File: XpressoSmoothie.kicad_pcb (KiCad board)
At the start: 2 copper layers, 99.7 x 99.7 mm, 129 parts, among them J1 HEADER_4, J10 HEADER_3X2, J11 Pwr_in, J12 HEADER_4, J13 HEADER_6, J14 HEADER_3X2, J15 HEADER_4, J16 HEADER_3, J17 HEADER_3, J18 HEADER_3, J19 HEADER_2, J2 HEADER_4, J20 HEADER_2, J21 HEADER_2, J22 HEADER_2, J23 HEADER_3, J24 HEADER_3, J25 HEADER_3, J26 USB, J27 HEADER_4, J28 MICROSD-MOLEX, J29 HEADER_4, J3 HEADER_3, J30 HEADER_4, J4 HEADER_3X2, J5 HEADER_3X2, J6 LPCXPRESSO_1769_HEADER, J7 HEADER_4, J8 HEADER_4, J9 HEADER_3X2, M1 LOGO_OSHW, M2 LOGO_OSHW, Q1 IRLB 8743, Q2 IRLB 8743, Q3 IRLB 8743, Q4 IRLB 8743, SW1 SW_PUSH, SW2 SW_PUSH, SW3 SW_PUSH, U1 POLOLU_A4988, U10 TC4422A, U11 TC4422A, U12 LM1117-3.3, U2 POLOLU_A4988, U3 POLOLU_A4988, U4 POLOLU_A4988, U5 POLOLU_A4988, U7 LM7809CT, U8 TC4422A, U9 TC4422A

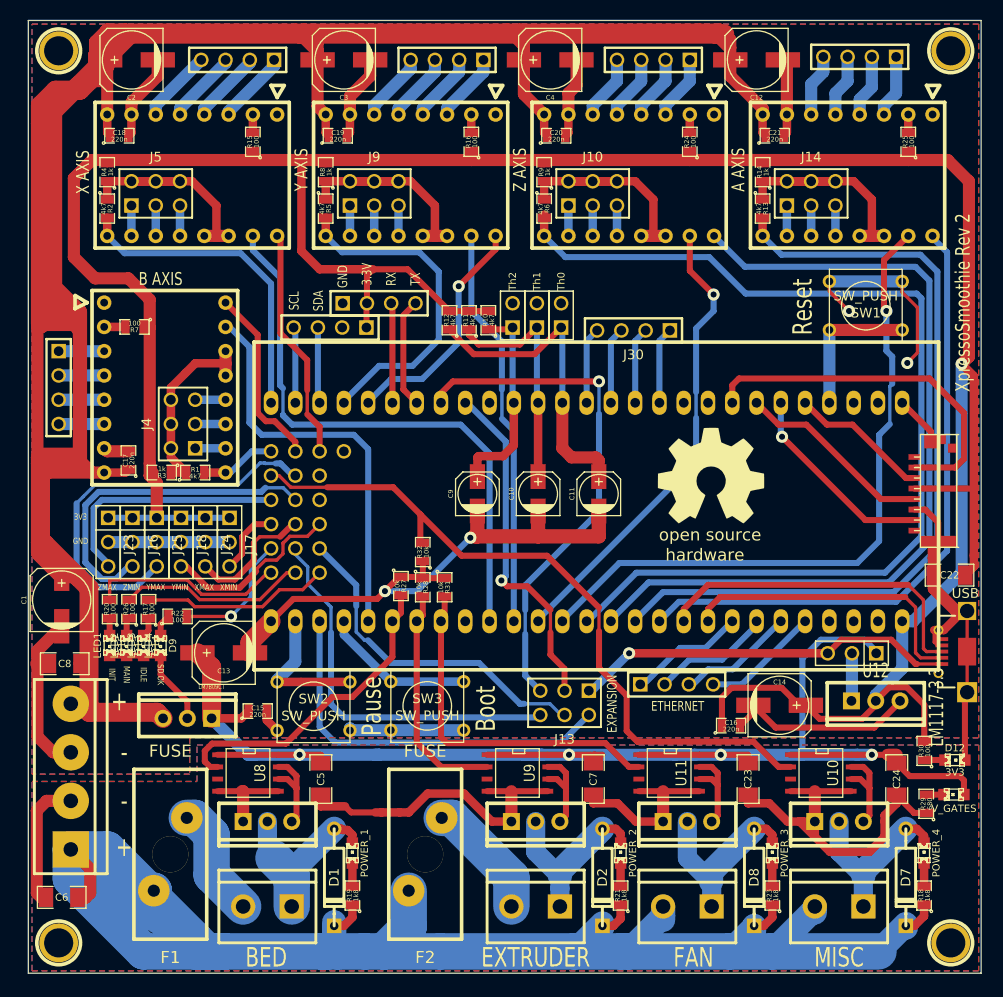
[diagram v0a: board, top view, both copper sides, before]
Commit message: Rev3 layout.
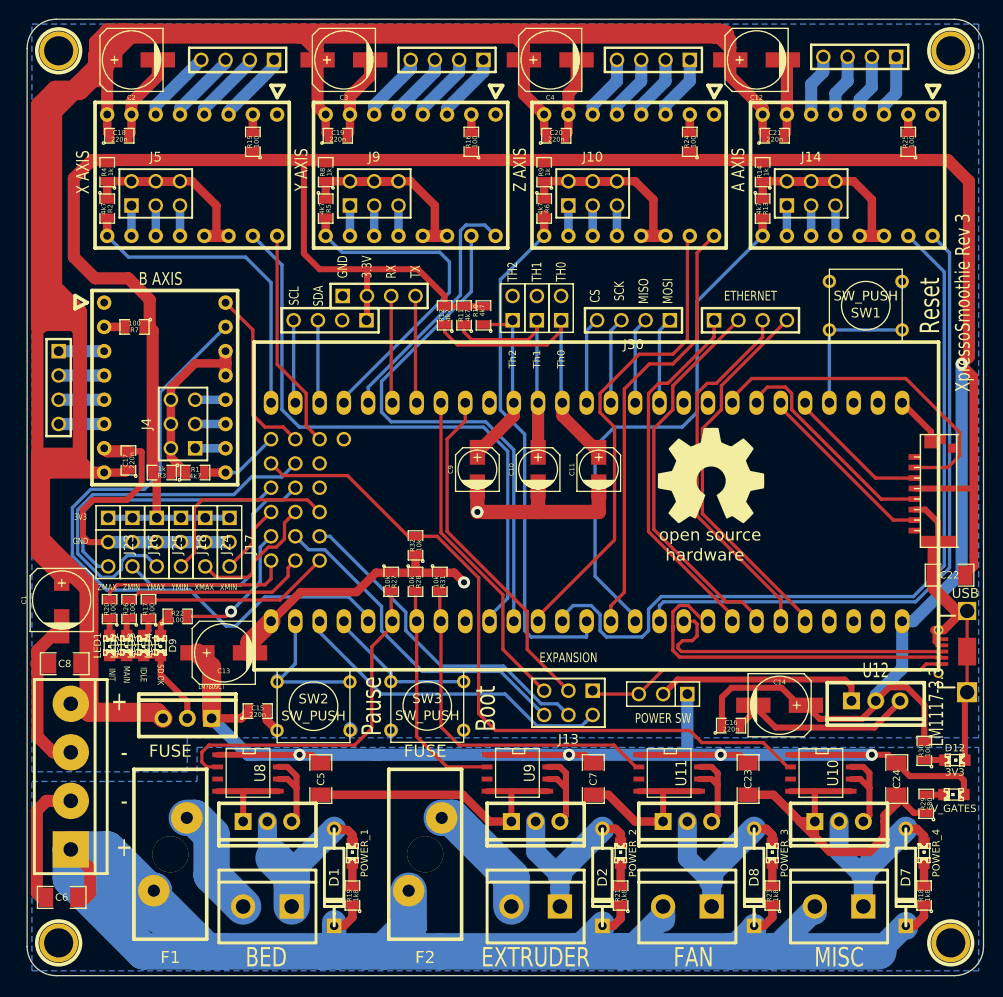
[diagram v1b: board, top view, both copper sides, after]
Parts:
- removed M1: LOGO_OSHW, OSHW_large_silkscreen-back_70mm
- moved J27 38.9 mm to (147.3, 85.3)
- moved J3 20.2 mm to (138.2, 124.5)
- moved C10 2.54 mm to (125.1, 101.0)
- moved C11 2.54 mm to (131.4, 101.0)
- moved C9 2.54 mm to (118.7, 101.0)
- moved R27 1.11 mm to (109.7, 112.7)
- moved J30 1.07 mm to (135.1, 85.3)
- moved R32 1.03 mm to (112.3, 108.9)
- moved R28 0.95 mm to (112.3, 112.7)
- moved R31 0.76 mm to (114.8, 112.7)
- moved J15 0.76 mm to (103.3, 85.3)
- moved J29 0.76 mm to (108.5, 82.8)
- moved Th0 0.76 mm to (127.5, 84.1)
- moved Th1 0.76 mm to (125.0, 84.1)
- moved Th2 0.76 mm to (122.4, 84.1)
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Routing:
- net Z-EN: track 108.0 -> 55.5 mm
- net Z-DIR: track 88.6 -> 46.7 mm
- net A-EN: track 85.6 -> 55.5 mm
- net B-STEP: track 42.9 -> 71.1 mm
- net *34_TD-: track 12.6 -> 40.6 mm
- net *32_RD-: track 12.4 -> 39.7 mm
- net *35_TD+: track 12.4 -> 39.3 mm
- net *33_RD+: track 12.4 -> 39.0 mm
- net GND: track 249.6 -> 225.6 mm, vias 4 -> 2
- net BUZZ: track 54.3 -> 34.6 mm, vias 1 -> 0
- net N-0000077: track 5.00 -> 22.2 mm
- net Vgates: track 162.6 -> 146.3 mm
- net Y-STEP: track 42.2 -> 55.7 mm
- net A-STEP: track 70.6 -> 83.9 mm, vias 1 -> 0
- net ZMIN: track 35.4 -> 25.6 mm
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- removed copper zone on F.Cu, net (none)
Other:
- board size 99.7 x 99.7 mm -> 100.1 x 100.1 mm
- board text added: "CS"
- board text added: "MISO"
- board text added: "MOSI"
- board text added: "POWER SW"
- board text added: "SCK"
- board text added: "TH0"
- board text added: "TH1"
- board text added: "TH2"
- board text added: "XpressoSmoothie Rev 3"
- board text removed: "XpressoSmoothie Rev 2"
